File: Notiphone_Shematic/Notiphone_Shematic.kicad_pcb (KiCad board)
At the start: 2 copper layers, 57.5 x 56 mm, 48 parts, among them J1 Conn_01x02_Pin, J2 USB_C_Receptacle_USB2.0_16P, M1 C0720B001F, Q1 2N3904, SW1 SW_Push, SW2 SW_Push, U1 AMS1117-3.3, U2 ESP32-S3-WROOM-1, U3 MCP73871, U4 INA333xxDGK

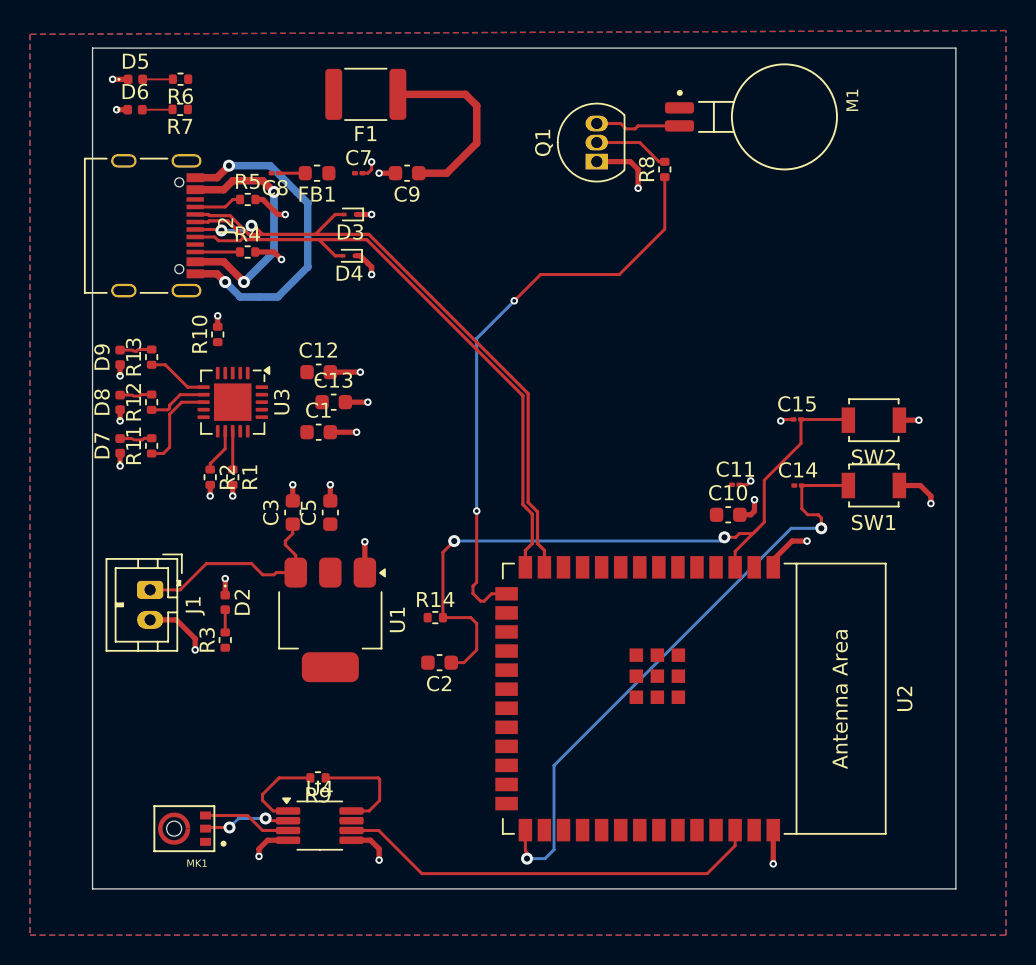
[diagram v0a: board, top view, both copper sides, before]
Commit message: Updated pcb file
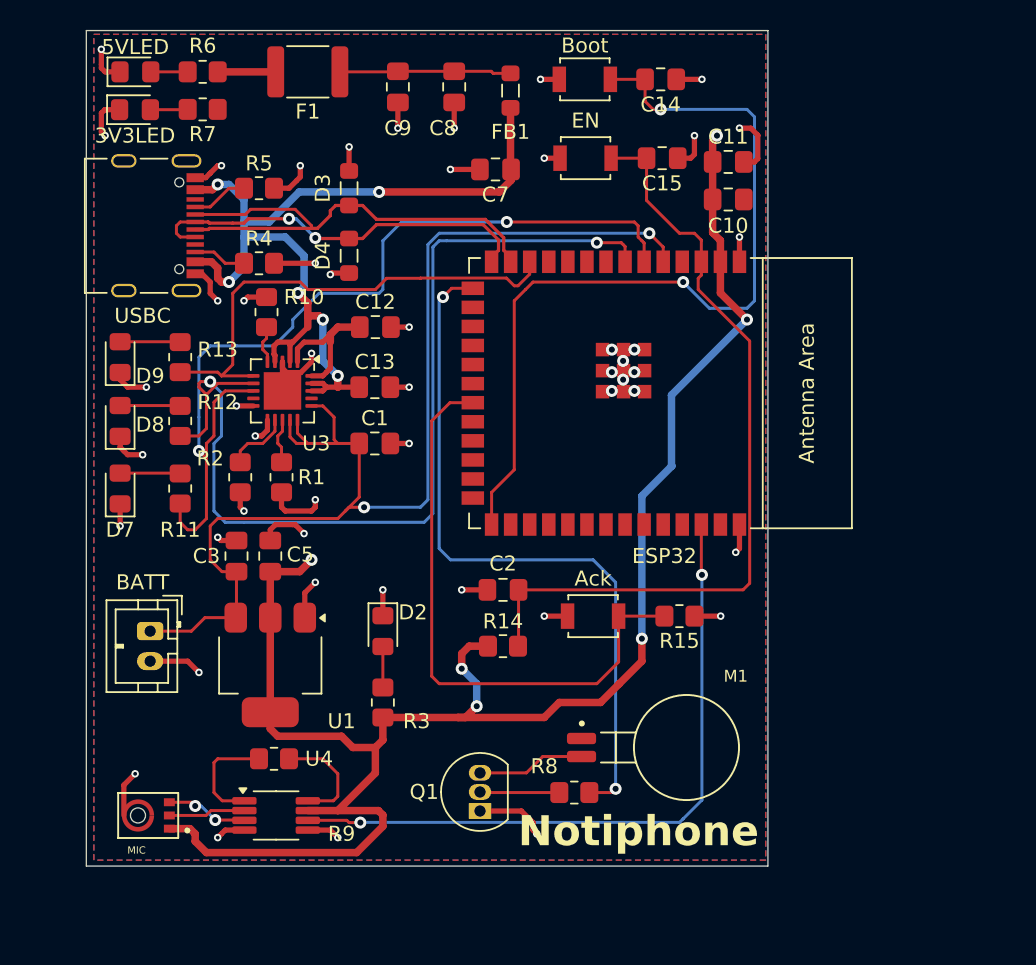
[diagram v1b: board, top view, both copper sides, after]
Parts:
- added Ack: ACK_BUTTON, Button_Switch_SMD:SW_SPST_B3U-1000P, F.Cu at (180.0, 61.2)
- added R15: 10k, Resistor_SMD:R_0805_2012Metric_Pad1.20x1.40mm_HandSolder, F.Cu at (185.8, 61.2)
- 3V3LED: renamed from D6; footprint LED_SMD:LED_0402_1005Metric -> LED_SMD:LED_0805_2012Metric_Pad1.15x1.40mm_HandSolder
- 5VLED: renamed from D5; footprint LED_SMD:LED_0402_1005Metric -> LED_SMD:LED_0805_2012Metric_Pad1.15x1.40mm_HandSolder
- Boot: renamed from SW1; value SW_Push -> Boot
- C1, C10, C12, C13, C2, C3, C5, C9: footprint Capacitor_SMD:C_0603_1608Metric -> Capacitor_SMD:C_0805_2012Metric_Pad1.18x1.45mm_HandSolder
- C11, C14, C15, C7, C8: footprint Capacitor_SMD:C_01005_0402Metric -> Capacitor_SMD:C_0805_2012Metric_Pad1.18x1.45mm_HandSolder
- D2, D7, D8, D9: footprint LED_SMD:LED_0402_1005Metric -> LED_SMD:LED_0805_2012Metric_Pad1.15x1.40mm_HandSolder
- D3, D4: footprint Diode_SMD:D_SOD-923 -> Inductor_SMD:L_0805_2012Metric_Pad1.05x1.20mm_HandSolder
- EN: renamed from SW2; value SW_Push -> EN
- FB1: footprint Inductor_SMD:L_0603_1608Metric -> Inductor_SMD:L_0805_2012Metric_Pad1.05x1.20mm_HandSolder
- R1, R10, R11, R12, R13, R14, R2, R3, R4, R5, R6, R7, R8, R9: footprint Resistor_SMD:R_0402_1005Metric -> Resistor_SMD:R_0805_2012Metric_Pad1.20x1.40mm_HandSolder
- moved Q1 43.9 mm to (172.5, 74.2)
- moved M1 42.5 mm to (184.2, 70.0)
- moved R8 41.9 mm to (178.8, 73.0), turned to 180 degrees
- moved Boot 33.2 mm to (179.4, 25.5), turned to 0 degrees
- moved C14 28.6 mm to (184.5, 25.5), turned to 180 degrees
- moved EN 25.9 mm to (179.5, 30.8), turned to 0 degrees
- moved C11 21.5 mm to (189.0, 31.0)
- moved C10 21.0 mm to (189.0, 33.5)
- moved ESP32 20.5 mm to (181.5, 46.4)
- moved C15 19.6 mm to (184.6, 30.8), turned to 180 degrees
- moved FB1 14.0 mm to (174.5, 26.2), turned to 90 degrees
- moved C8 13.2 mm to (170.8, 26.0), turned to -90 degrees
- moved R3 11.3 mm to (166.0, 67.0)
- moved D2 10.7 mm to (166.0, 62.2)
- moved C7 9.11 mm to (173.5, 31.5), turned to 180 degrees
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- renumbered J1 to BATT, U2 to ESP32, MK1 to MIC, J2 to USBC
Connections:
- ESP32 pad 21: unconnected-(U2-GPIO13/TOUCH13/ADC2_CH2/FSPIQ/FSPIIO7/SUBSPIQ-Pad21) -> GPIO_A13
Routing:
- net VCC_3V3: track 0.00 -> 115.5 mm, vias 0 -> 6
- net GPIO_A5: track 14.5 -> 79.3 mm, vias 0 -> 2
- net CHRG_COMPLETE: track 4.00 -> 65.6 mm, vias 0 -> 2
- net CHRGING_LED: track 6.17 -> 59.5 mm, vias 0 -> 2
- net PWRU_IN: track 16.4 -> 62.0 mm, vias 2 -> 6
- net GPIO_A13: track 0.00 -> 39.6 mm
- net GPIO_A8: track 4.08 -> 32.8 mm
- net USBC_D.P: track 44.0 -> 26.6 mm, vias 0 -> 2
- net GND: track 75.8 -> 92.8 mm, vias 34 -> 50
- net GPIO_A2: track 28.5 -> 45.3 mm, vias 0 -> 2
- net BOOT: track 40.8 -> 56.7 mm
- net USBC_D.N: track 46.5 -> 32.6 mm, vias 2 -> 0
- net V_SYSTEM: track 0.00 -> 9.33 mm
- net GPIO_A3: track 38.8 -> 47.4 mm
- net EN: track 47.0 -> 53.6 mm, vias 2 -> 0
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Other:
- board size 57.5 x 56 mm -> 45.4 x 55.6 mm
- board text added: "Notiphone"
